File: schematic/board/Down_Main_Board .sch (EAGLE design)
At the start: 26 parts, among them J1 MCX-J-P-H-ST-TH1, J2 U.FL-R-SMT-1_10_

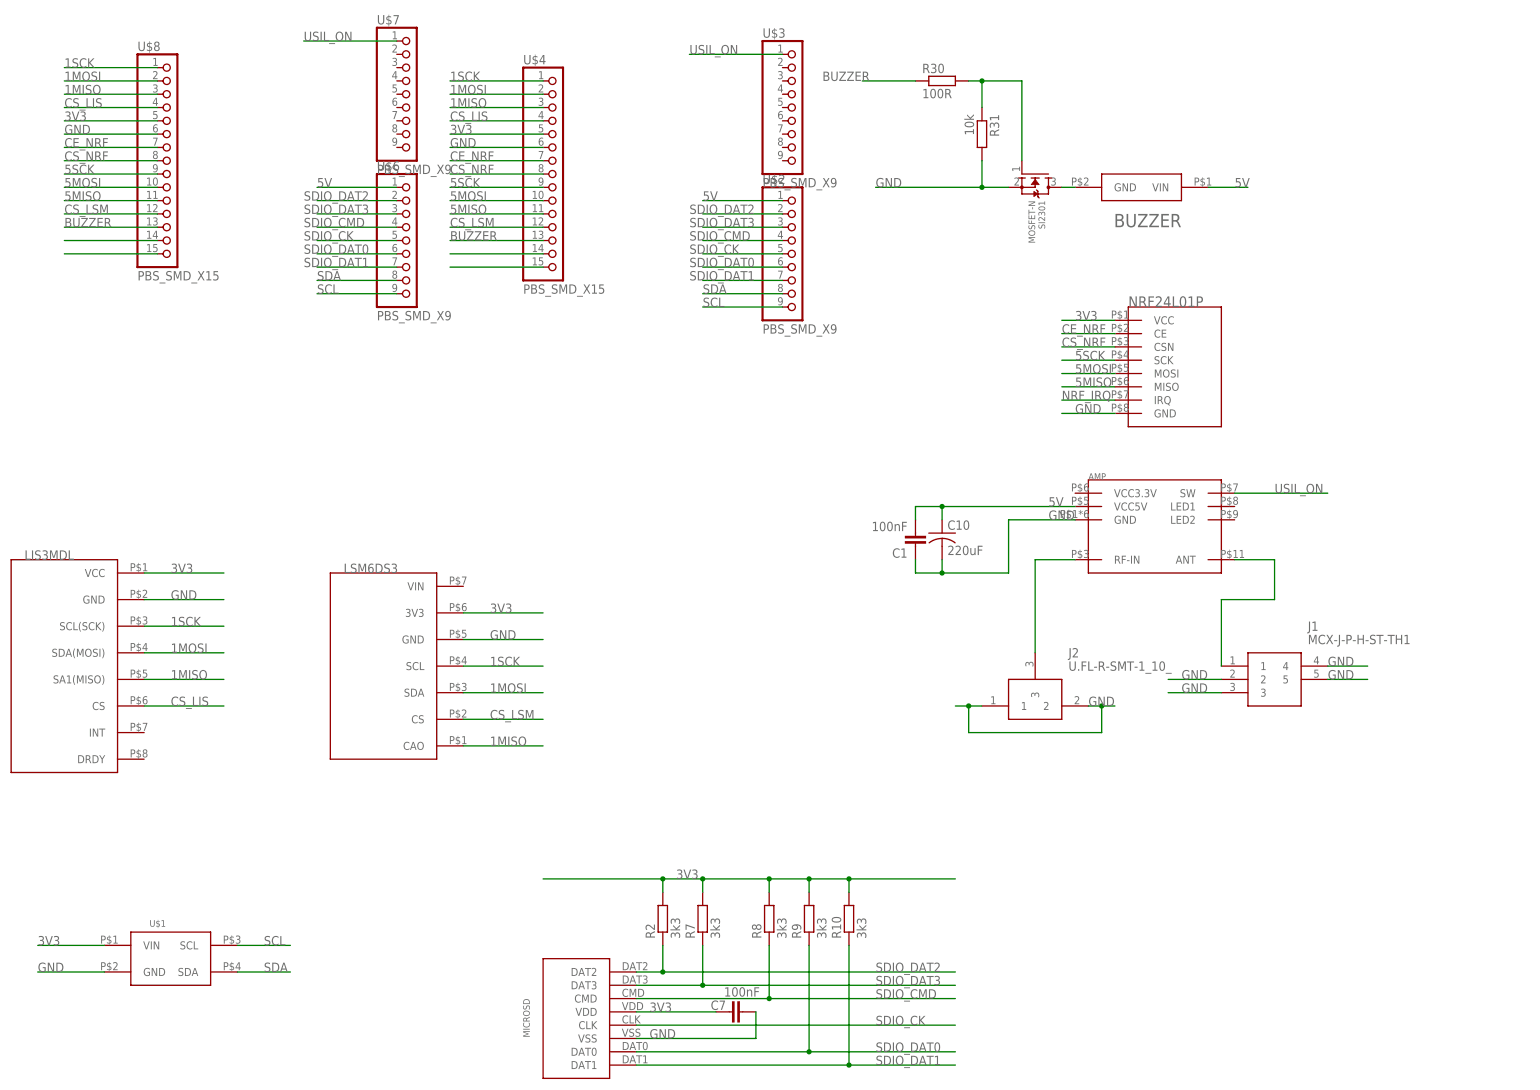
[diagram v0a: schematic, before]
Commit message: Почти доделал нижнюю плату
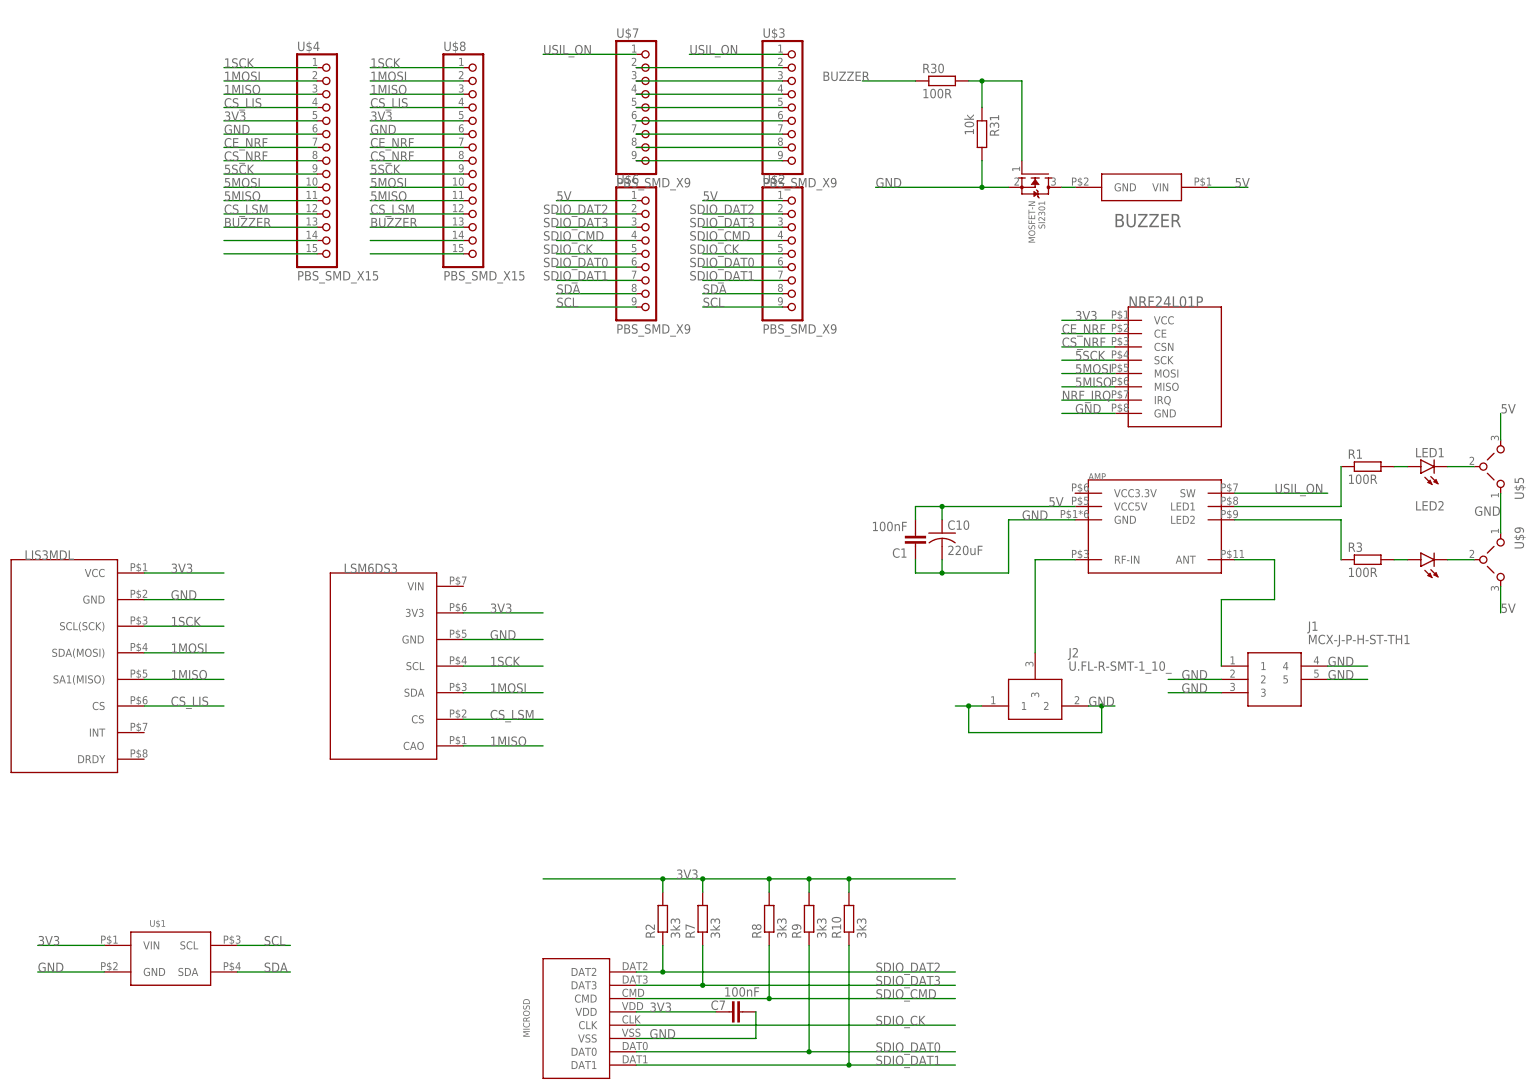
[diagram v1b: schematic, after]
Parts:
- added LED1, LED2: (no value), led:LEDCHIPLED_0603
- added R1, R3: 100R, rcl:R-EU_R0603
- added U$5, U$9: VIAS-SELECT, NEON-BLADE-2024:VIAS-SELECT
- LIS3MDL: value LIS3MDL-CJMCUБез_отв._зеркальный -> LIS3MDL-CJMCUбез_отв.; device NEON-BLADE-2023:LIS3MDL-CJMCUБез_отв._зеркальный -> NEON-BLADE-2023:LIS3MDL-CJMCUбез_отв.
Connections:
- new net N$10: U$3.6, U$7.6
- new net N$11: U$3.7, U$7.7
- new net N$14: U$3.8, U$7.8
- new net N$15: U$3.9, U$7.9
- new net N$16: LED1.C, U$5.TOP
- new net N$17: LED1.A, R1.2
- new net N$18: AMP.LED1, R1.1
- new net N$19: LED2.C, U$9.TOP
- new net N$21: LED2.A, R3.2
- new net N$22: AMP.LED2, R3.1
- new net N$6: U$3.2, U$7.2
- new net N$7: U$3.3, U$7.3
- new net N$8: U$3.4, U$7.4
- new net N$9: U$3.5, U$7.5
- net 5V: now also U$5.RIGHT, U$9.RIGHT
- net GND: now also U$5.LEFT, U$9.LEFT
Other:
- moved on the sheet: U$4, U$6, U$7, U$8
